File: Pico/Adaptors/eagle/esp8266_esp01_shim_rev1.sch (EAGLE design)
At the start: 4 parts, among them IC1 LD117AS33TR

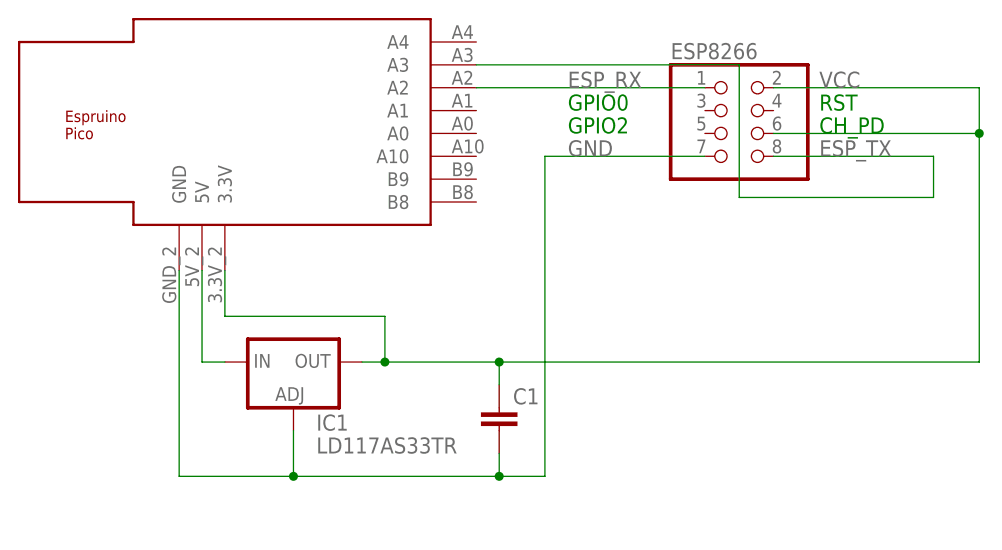
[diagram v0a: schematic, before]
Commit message: tweak net classes
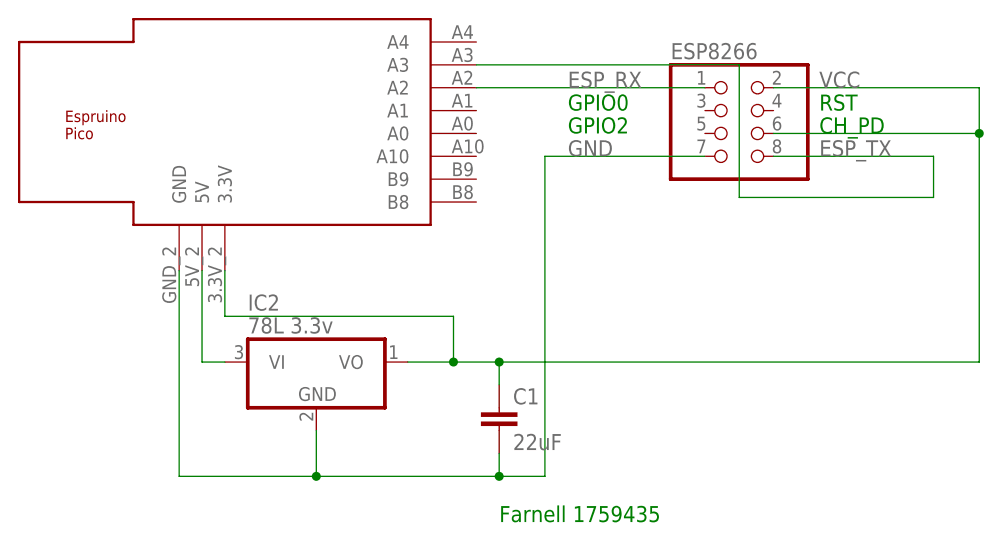
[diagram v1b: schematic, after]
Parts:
- removed IC1: LD117AS33TR, v-reg:LD117AS33TR
- added IC2: 78L 3.3v, linear:78L05Z
- C1: value (none) -> 22uF
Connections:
- net GND: now also IC2.GND; no longer IC1.ADJ
- net N$1: now also IC2.VI; no longer IC1.IN
- net VCC: now also IC2.VO; no longer IC1.OUT
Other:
- note added: "Farnell 1759435"
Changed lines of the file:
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@@
 </variantdefs>
 <classes>
-<class number="0" name="default" width="0" drill="0">
+<class number="0" name="default" width="0.3048" drill="0">
 </class>
 </classes>
 <parts>
 <part name="ESP8266" library="pinhead" deviceset="PINHD-2X4" device=""/>
-<part name="IC1" library="v-reg" deviceset="LD117A?*" device="S" technology="33TR"/>
-<part name="C1" library="rcl" deviceset="C-EU" device="C1210"/>
+<part name="C1" library="rcl" deviceset="C-EU" device="C1210" value="22uF"/>
 <part name="U$1" library="espruino_pico" deviceset="ESPRUINO_PICO_0.05" device=""/>
+<part name="IC2" library="linear" deviceset="78*" device="Z" technology="L05" value="78L 3.3v"/>
 </parts>
 <sheets>
@@
 <text x="78.74" y="43.18" size="1.778" layer="91">GPIO0</text>
 <text x="78.74" y="40.64" size="1.778" layer="91">GPIO2</text>
+<text x="71.12" y="-2.54" size="1.778" layer="91">Farnell 1759435</text>
 </plain>
 <instances>
 <instance part="ESP8266" gate="A" x="96.52" y="40.64"/>
-<instance part="IC1" gate="G$1" x="48.26" y="15.24"/>
 <instance part="C1" gate="G$1" x="71.12" y="10.16"/>
 <instance part="U$1" gate="G$1" x="50.8" y="43.18"/>
+<instance part="IC2" gate="A1" x="50.8" y="15.24"/>
 </instances>
 <busses>
@@
 <wire x1="101.6" y1="45.72" x2="124.46" y2="45.72" width="0.1524" layer="91"/>
 <wire x1="124.46" y1="45.72" x2="124.46" y2="40.64" width="0.1524" layer="91"/>
-<pinref part="IC1" gate="G$1" pin="OUT"/>
 <wire x1="124.46" y1="40.64" x2="124.46" y2="15.24" width="0.1524" layer="91"/>
 <wire x1="124.46" y1="15.24" x2="71.12" y2="15.24" width="0.1524" layer="91"/>
-<wire x1="71.12" y1="15.24" x2="58.42" y2="15.24" width="0.1524" layer="91"/>
-<wire x1="58.42" y1="15.24" x2="55.88" y2="15.24" width="0.1524" layer="91"/>
+<wire x1="71.12" y1="15.24" x2="66.04" y2="15.24" width="0.1524" layer="91"/>
+<wire x1="66.04" y1="15.24" x2="60.96" y2="15.24" width="0.1524" layer="91"/>
 <wire x1="40.64" y1="25.4" x2="40.64" y2="20.32" width="0.1524" layer="91"/>
-<wire x1="40.64" y1="20.32" x2="58.42" y2="20.32" width="0.1524" layer="91"/>
-<wire x1="58.42" y1="20.32" x2="58.42" y2="15.24" width="0.1524" layer="91"/>
+<wire x1="40.64" y1="20.32" x2="66.04" y2="20.32" width="0.1524" layer="91"/>
+<wire x1="66.04" y1="20.32" x2="66.04" y2="15.24" width="0.1524" layer="91"/>
 <label x="106.68" y="45.72" size="1.778" layer="95"/>
 <pinref part="ESP8266" gate="A" pin="6"/>
@@
 <pinref part="C1" gate="G$1" pin="1"/>
 <wire x1="71.12" y1="15.24" x2="71.12" y2="12.7" width="0.1524" layer="91"/>
-<junction x="58.42" y="15.24"/>
+<junction x="66.04" y="15.24"/>
 <junction x="71.12" y="15.24"/>
 <pinref part="U$1" gate="G$1" pin="3.3V"/>
+<pinref part="IC2" gate="A1" pin="VO"/>
 </segment>
 </net>
@@
 <segment>
 <wire x1="35.56" y1="25.4" x2="35.56" y2="2.54" width="0.1524" layer="91"/>
-<wire x1="35.56" y1="2.54" x2="48.26" y2="2.54" width="0.1524" layer="91"/>
-<pinref part="IC1" gate="G$1" pin="ADJ"/>
-<wire x1="48.26" y1="2.54" x2="48.26" y2="7.62" width="0.1524" layer="91"/>
-<wire x1="48.26" y1="2.54" x2="71.12" y2="2.54" width="0.1524" layer="91"/>
+<wire x1="35.56" y1="2.54" x2="50.8" y2="2.54" width="0.1524" layer="91"/>
+<wire x1="50.8" y1="2.54" x2="50.8" y2="7.62" width="0.1524" layer="91"/>
+<wire x1="50.8" y1="2.54" x2="71.12" y2="2.54" width="0.1524" layer="91"/>
 <wire x1="71.12" y1="2.54" x2="76.2" y2="2.54" width="0.1524" layer="91"/>
 <wire x1="76.2" y1="2.54" x2="76.2" y2="38.1" width="0.1524" layer="91"/>
@@
 <wire x1="71.12" y1="5.08" x2="71.12" y2="2.54" width="0.1524" layer="91"/>
 <junction x="71.12" y="2.54"/>
-<junction x="48.26" y="2.54"/>
+<junction x="50.8" y="2.54"/>
 <pinref part="U$1" gate="G$1" pin="GND"/>
+<pinref part="IC2" gate="A1" pin="GND"/>
 </segment>
 </net>
@@
 <segment>
 <wire x1="38.1" y1="25.4" x2="38.1" y2="15.24" width="0.1524" layer="91"/>
-<pinref part="IC1" gate="G$1" pin="IN"/>
 <wire x1="38.1" y1="15.24" x2="40.64" y2="15.24" width="0.1524" layer="91"/>
 <pinref part="U$1" gate="G$1" pin="5V"/>
+<pinref part="IC2" gate="A1" pin="VI"/>
 </segment>
 </net>
